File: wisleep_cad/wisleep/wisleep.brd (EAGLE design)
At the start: 52.4 x 54.3 mm, 55 parts, among them IC1 STM32F10XCXT6, X1 8MHz, X2 32kHz

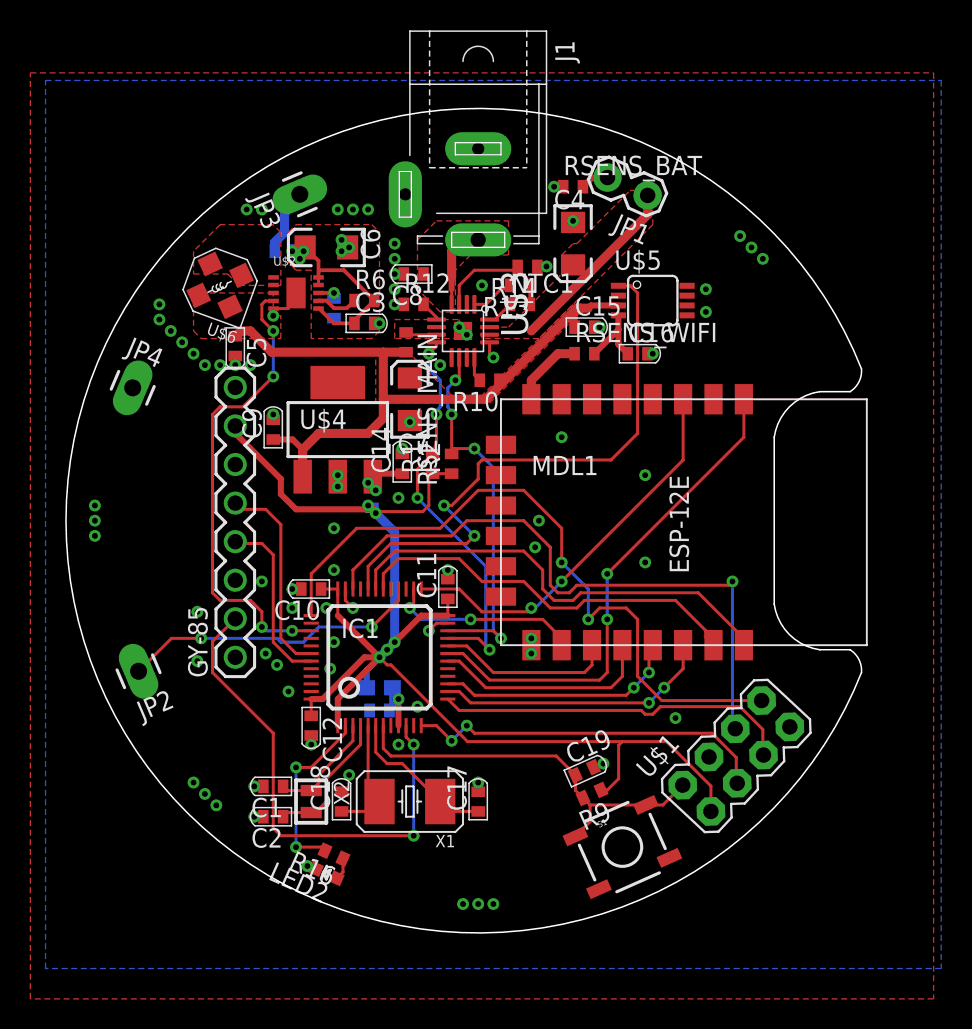
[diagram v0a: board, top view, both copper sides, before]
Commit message: wisleep cad rev A - 2 fab
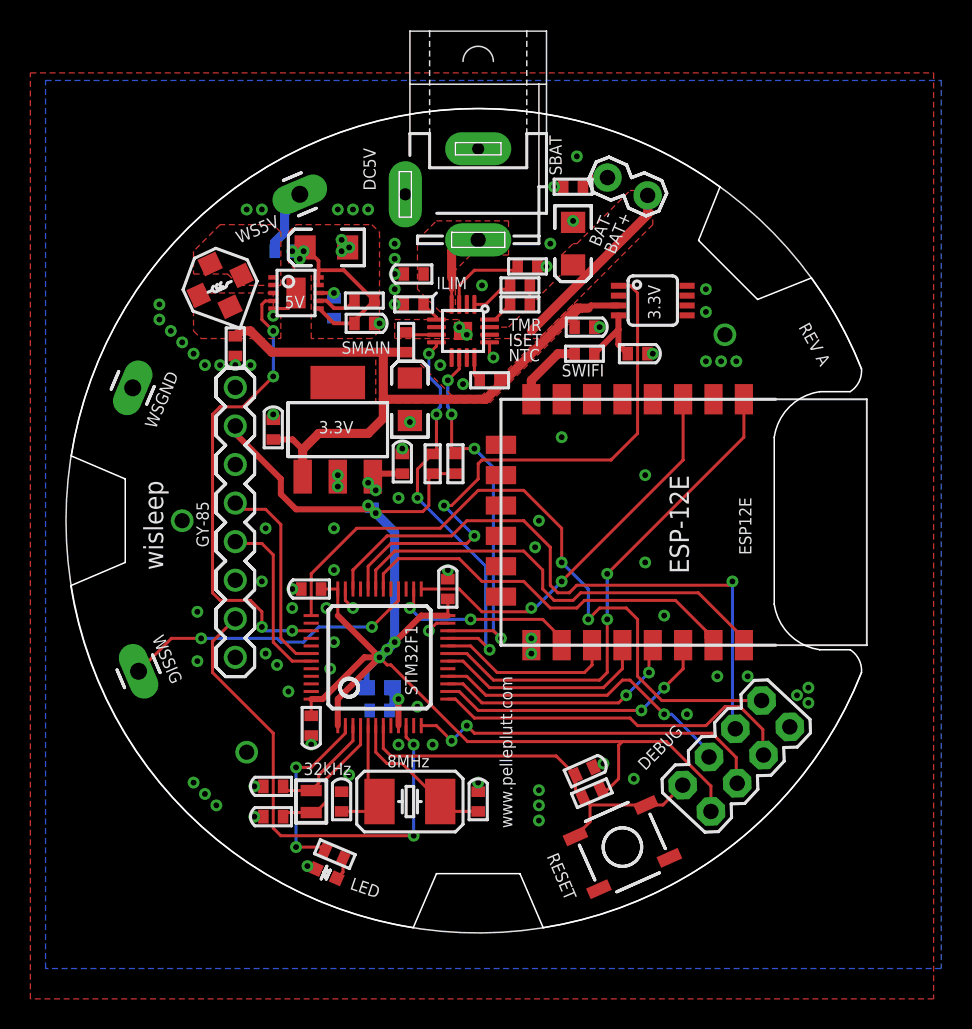
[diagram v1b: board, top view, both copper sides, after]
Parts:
- moved U$7 54.6 mm to (45.4, 40.8)
- moved R2 0.25 mm to (25.5, 30.8)
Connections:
- removed net N$18: IC1.16
- removed net N$7: U$1.4
- new net DBG_IO: IC1.16, U$1.4
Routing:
- net DBG_IO: track 0.00 -> 20.4 mm, vias 0 -> 1
- net WIFI_IO5: track 18.3 -> 19.1 mm
- net USART_RX: track 23.7 -> 24.3 mm
- net GND: track 8.27 -> 8.75 mm, vias 87 -> 99
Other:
- board size 52.4 x 54.3 mm -> 52.1 x 54 mm
- board text added: "3.3V"
- board text added: "32kHz"
- board text added: "5V"
- board text added: "8MHz"
- board text added: "BAT+"
- board text added: "BAT-"
- board text added: "DC5V"
- board text added: "DEBUG"
- board text added: "ESP12E"
- board text added: "GY-85"
- board text added: "ILIM"
- board text added: "ISET"
- board text added: "LED"
- board text added: "NTC"
- board text added: "RESET"
- board text added: "REV A"
- board text added: "S5V"
- board text added: "SBAT"
- board text added: "SCPU"
- board text added: "SMAIN"
- board text added: "STM32F1"
- board text added: "SWIFI"
- board text added: "TMR"
- board text added: "WS5V"
- board text added: "WSGND"
- board text added: "WSSIG"
- board text added: "wisleep"
- board text added: "www.pelleplutt.com"
